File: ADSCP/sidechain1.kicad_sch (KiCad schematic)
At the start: 7 parts, among them U4 TL074

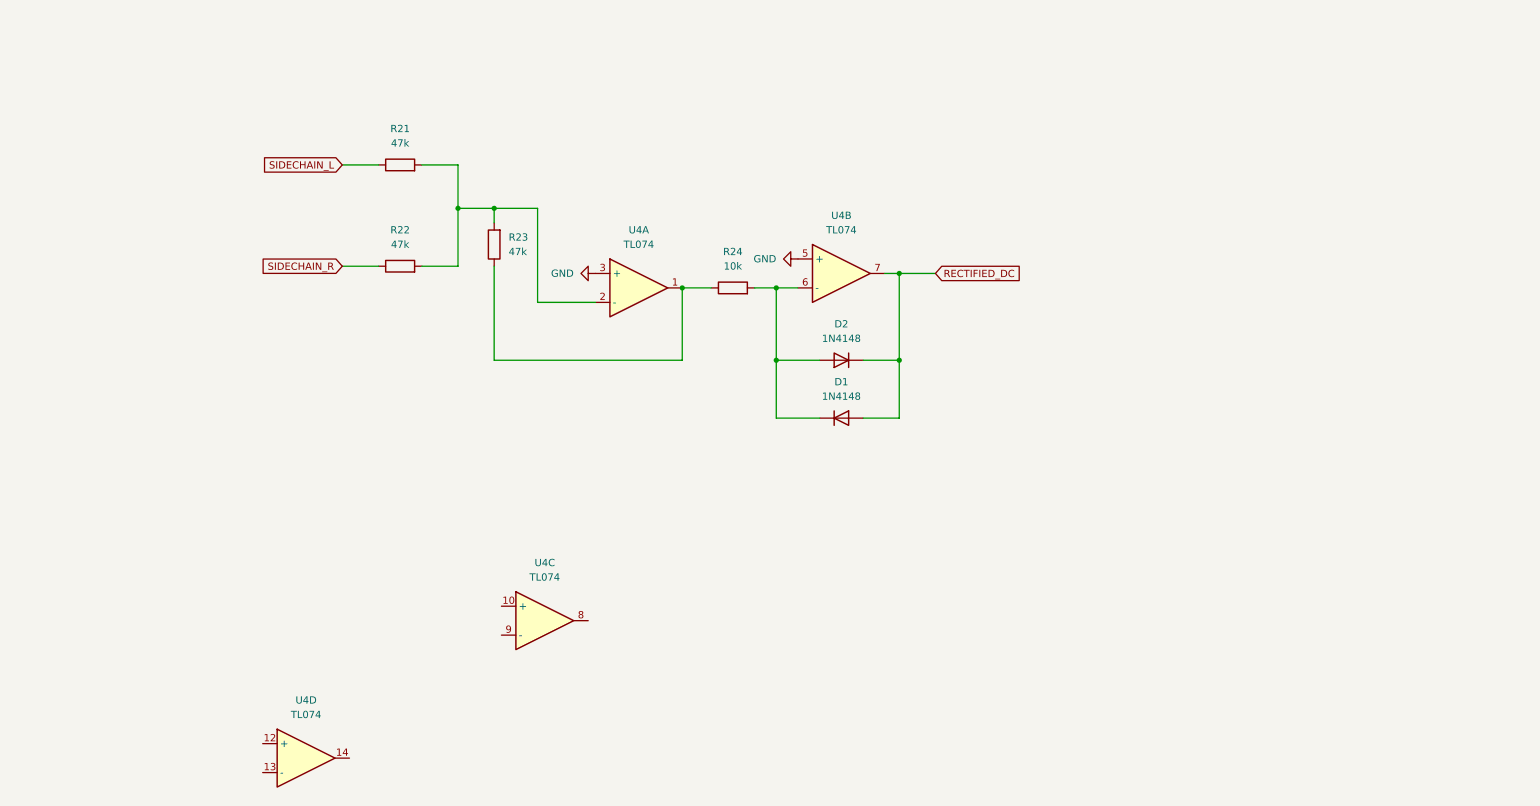
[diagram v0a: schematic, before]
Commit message: add schematics
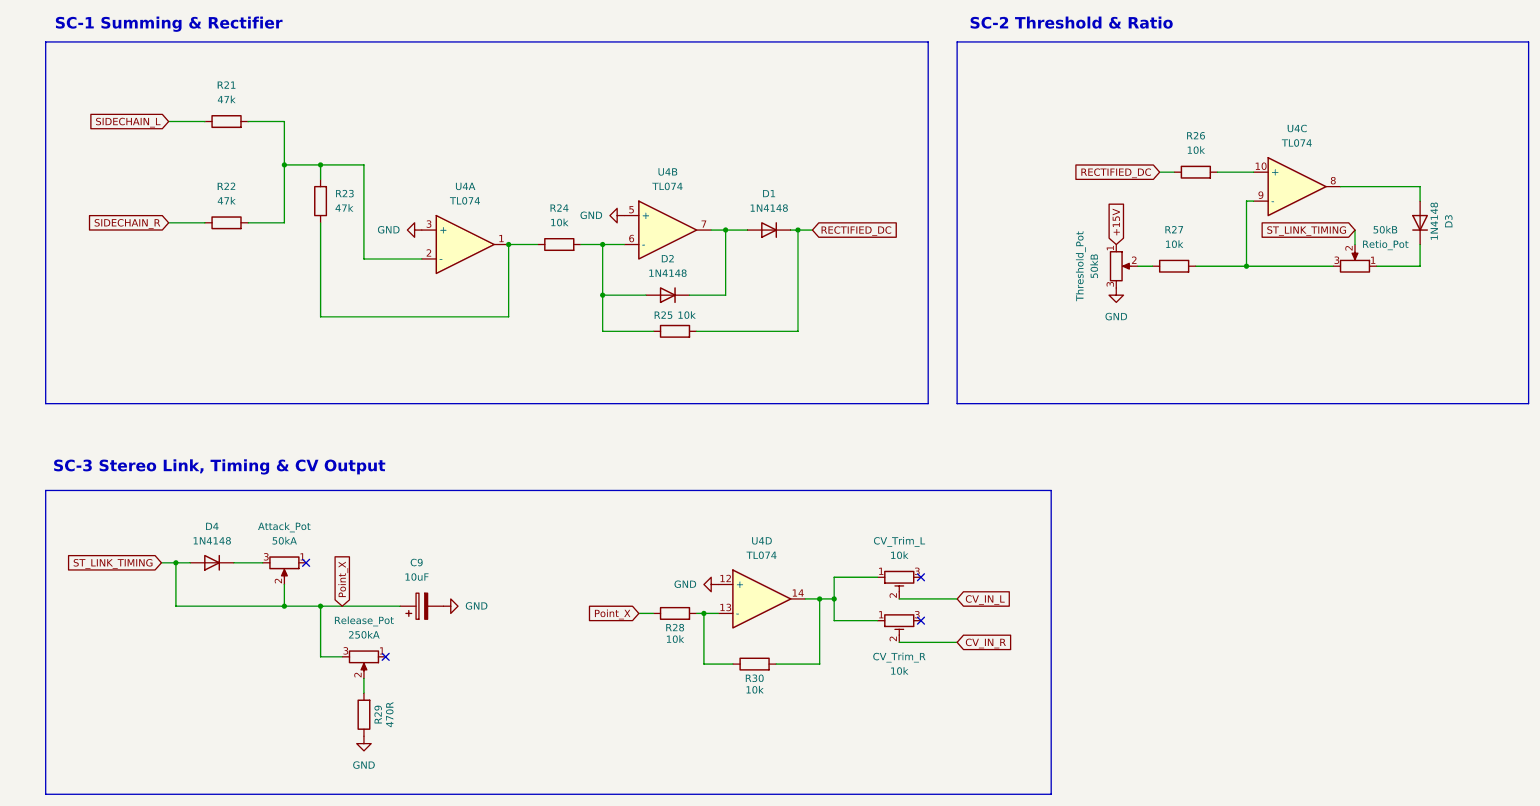
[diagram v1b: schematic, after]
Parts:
- added Attack_Pot: 50kA, Connector_PinHeader_2.54mm:PinHeader_1x03_P2.54mm_Vertical, symbol Device:R_Potentiometer
- added C9: 10uF, Capacitor_THT:CP_Radial_D8.0mm_P3.50mm, symbol Device:C_Polarized
- added CV_Trim_L, CV_Trim_R: 10k, Potentiometer_THT:Potentiometer_Runtron_RM-065_Vertical, symbol Device:R_Potentiometer_Trim
- added D3, D4: 1N4148, Diode_THT:D_DO-35_SOD27_P7.62mm_Horizontal, symbol Device:D
- added R25, R26, R27, R28, R30: 10k, Resistor_THT:R_Axial_DIN0207_L6.3mm_D2.5mm_P2.54mm_Vertical, symbol Device:R
- added R29: 470R, Resistor_THT:R_Axial_DIN0207_L6.3mm_D2.5mm_P2.54mm_Vertical, symbol Device:R
- added Release_Pot: 250kA, Connector_PinHeader_2.54mm:PinHeader_1x03_P2.54mm_Vertical, symbol Device:R_Potentiometer
- added Retio_Pot, Threshold_Pot: 50kB, Connector_PinHeader_2.54mm:PinHeader_1x03_P2.54mm_Vertical, symbol Device:R_Potentiometer
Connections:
- net GND: now also U4.12 (+), C9.2, R29.1, Threshold_Pot.3
- net RECTIFIED_DC: now also D1.1 (K), R25.2, R26.1; no longer D1.2 (A), D2.1 (K), U4.7
- net at U4.13 (-): now also R28.2, R30.1
- net at U4.14: now also CV_Trim_L.1, CV_Trim_R.1, R30.2
- net at D2.2 (A), R24.2, U4.6 (-): now also R25.1; no longer D1.1 (K)
- net at U4.10 (+): now also R26.2
- net at U4.8: now also D3.2 (A)
- net at U4.9 (-): now also R27.2, Retio_Pot.3
- new net: Attack_Pot.3, D4.1 (K)
- new net: D1.2 (A), D2.1 (K), U4.7
- new net: D3.1 (K), Retio_Pot.1
- new net: R27.1, Threshold_Pot.2
- new net: R29.2, Release_Pot.2
- new net +15V: Threshold_Pot.1
- new net CV_IN_L: CV_Trim_L.2
- new net CV_IN_R: CV_Trim_R.2
- new net Point_X: Attack_Pot.2, C9.1, D4.2 (A), R28.1, Release_Pot.3, Retio_Pot.2
- no-connect marks 0 -> 4
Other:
- note added: "SC-1 Summing & Rectifier"
- note added: "SC-2 Threshold & Ratio"
- note added: "SC-3 Stereo Link, Timing & CV Output"
- moved on the sheet: D1, D2, R21, R22, R23, R24, U4A, U4B, U4C, U4D

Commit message: add schematics
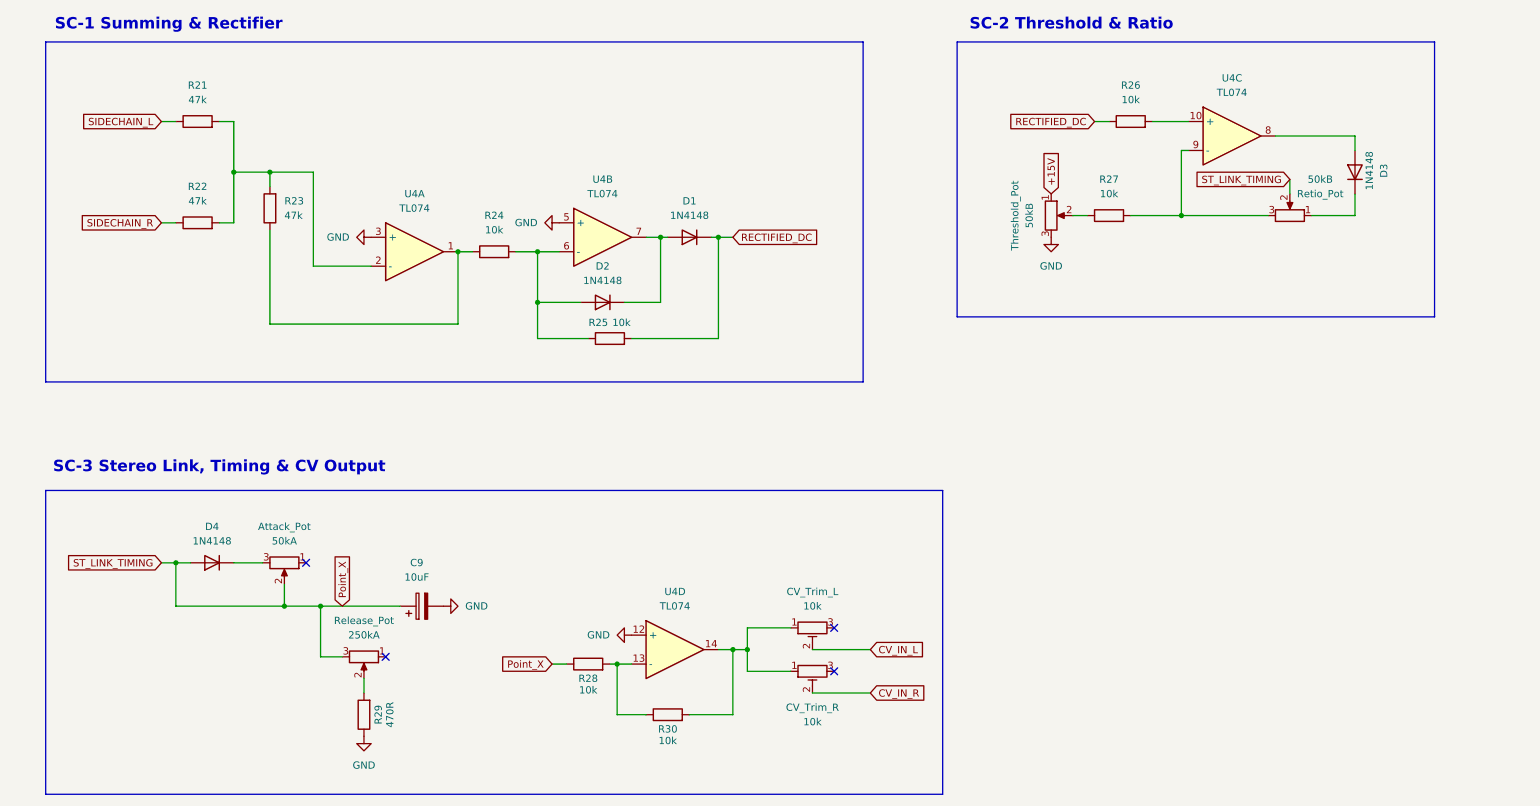
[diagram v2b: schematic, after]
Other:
- moved on the sheet: CV_Trim_L, CV_Trim_R, D1, D2, D3, R21, R22, R23, R24, R25, R26, R27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
